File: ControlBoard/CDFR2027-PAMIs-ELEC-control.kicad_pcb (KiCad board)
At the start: 4 copper layers, 96.8 x 76.6 mm, 92 parts, among them J1 Conn_01x04_Pin, Q1 PMOS, U1 USBLC6-2P6

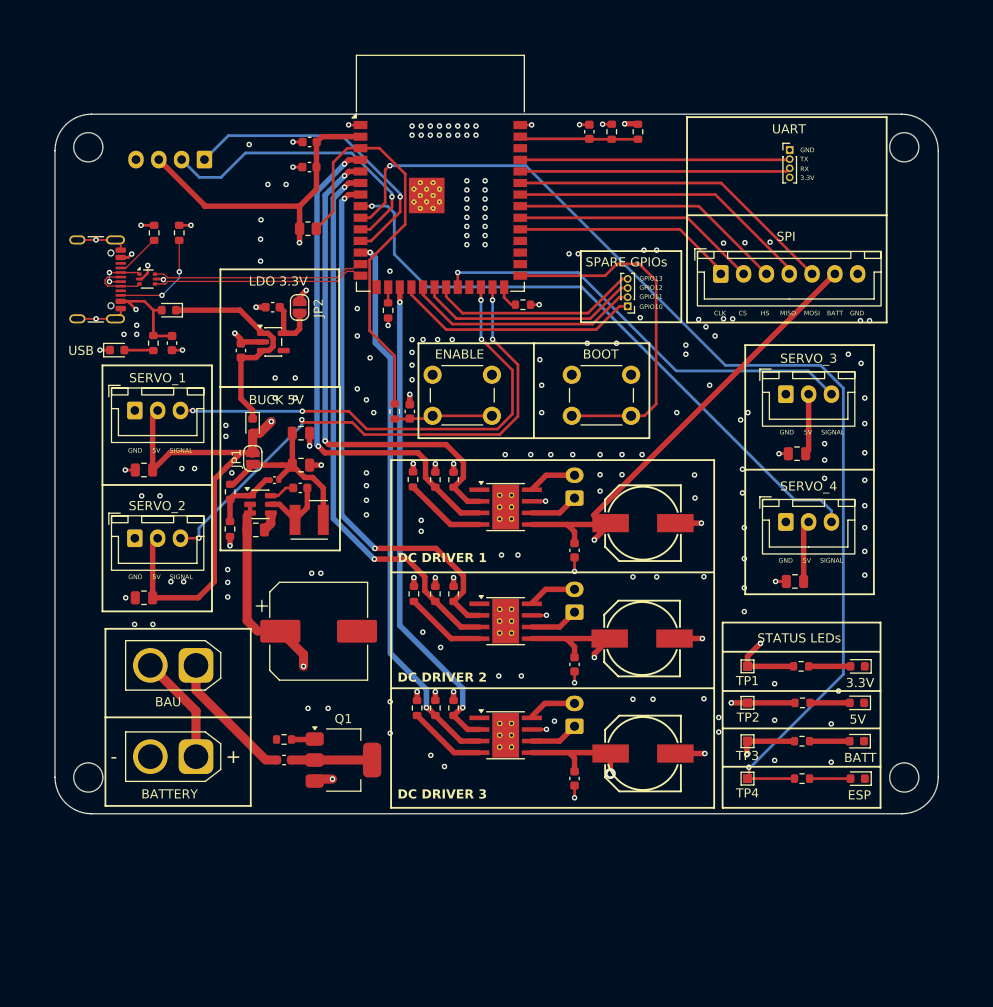
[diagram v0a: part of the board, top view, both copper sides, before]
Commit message: (feat): routing v2
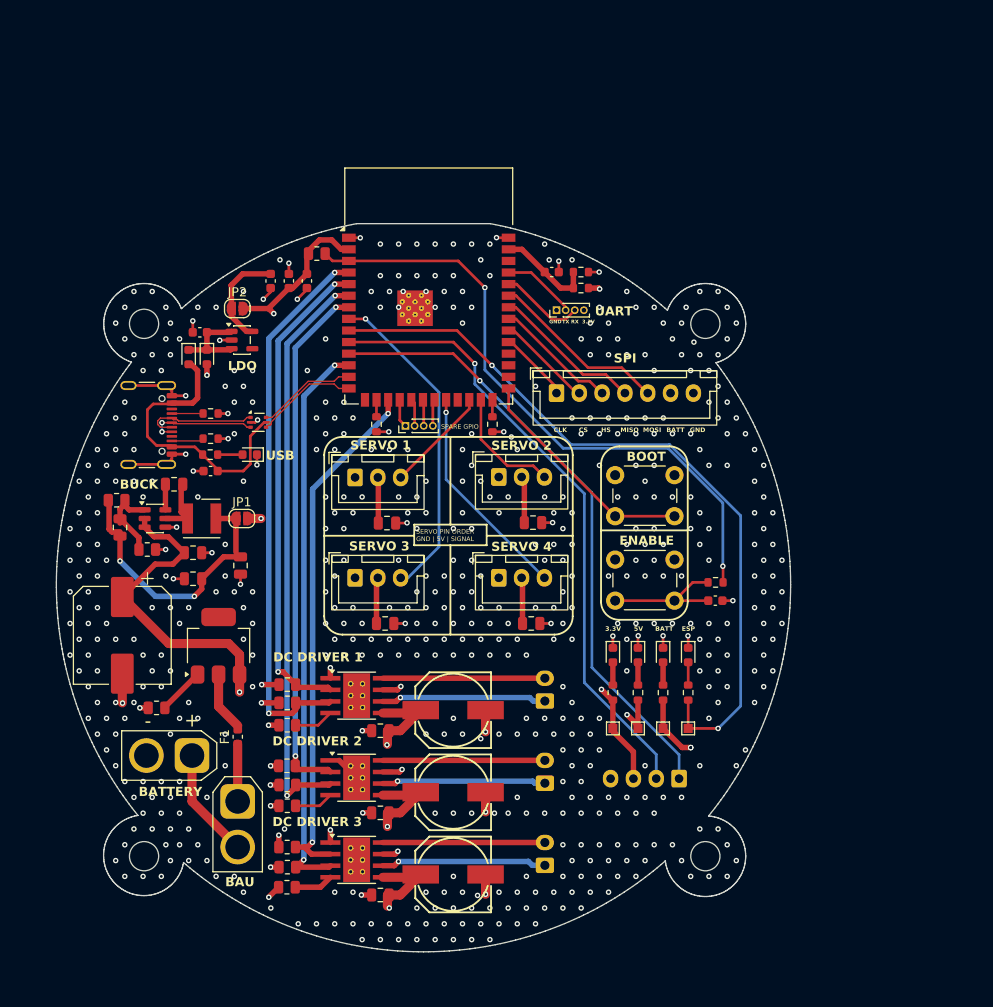
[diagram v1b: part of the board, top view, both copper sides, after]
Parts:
- C13, C15, C17, C7: footprint Capacitor_SMD:C_0603_1608Metric -> Capacitor_SMD:C_0805_2012Metric
- C19: footprint Capacitor_SMD:C_0402_1005Metric -> Capacitor_SMD:C_0805_2012Metric
- R10, R11, R12, R13, R14, R15, R16, R17, R5, R9: footprint Resistor_SMD:R_0603_1608Metric -> Resistor_SMD:R_0805_2012Metric
- R18, R19: footprint PCM_SparkFun-Resistor:R_0603_1608Metric -> Resistor_SMD:R_0805_2012Metric
- moved H4 97.0 mm to (93.6, 85.7)
- moved I2C1 85.5 mm to (152.2, 135.5)
- moved H3 83.9 mm to (155.1, 85.7)
- moved H2 80.7 mm to (155.1, 144.0)
- moved H1 77.9 mm to (93.6, 144.0)
- moved SERVO_4 47.6 mm to (116.8, 113.5)
- moved C23 45.1 mm to (120.0, 118.5), turned to 0 degrees
- moved REF** 43.7 mm to (124.5, 108.6)
- moved C21 43.4 mm to (136.2, 107.5), turned to 0 degrees
- moved SERVO_2 40.4 mm to (132.5, 102.5)
- moved R1 39.8 mm to (156.2, 114.0), turned to 0 degrees
- moved C1 39.4 mm to (156.2, 116.0), turned to 180 degrees
- moved SERVO_3 37.3 mm to (132.5, 113.5)
- moved C22 34.6 mm to (136.1, 118.5), turned to 0 degrees
- moved UART1 31.0 mm to (138.8, 84.2), turned to 90 degrees
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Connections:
- net Net-(U1-I/O1-Pad1) renamed /External IO/D-
- net Net-(U1-I/O2-Pad3) renamed /External IO/D+
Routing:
- net +3.3V: track 179.3 -> 106.9 mm, vias 3 -> 2
- net BATT: track 310.3 -> 245.7 mm
- net +5V: track 176.1 -> 119.9 mm, vias 2 -> 3
- net /Actuators & Utility/SERVO_2: track 60.4 -> 13.0 mm, vias 4 -> 0
- net /Actuators & Utility/SERVO_1: track 53.2 -> 11.6 mm, vias 4 -> 0
- net /Actuators & Utility/STATUS_LED: track 119.6 -> 82.1 mm
- net /External IO/SDA: track 32.7 -> 68.5 mm
- net /External IO/SCL: track 32.8 -> 68.2 mm
- net /Actuators & Utility/SERVO_4: track 69.3 -> 35.7 mm
- net /Actuators & Utility/SERVO_3: track 48.1 -> 24.0 mm
- net /Actuators & Utility/GPIO10: track 27.2 -> 3.11 mm
- net /Actuators & Utility/GPIO11: track 26.3 -> 3.00 mm
- net Net-(ESP32-S3-WROOM1-EN): track 45.9 -> 68.9 mm, vias 0 -> 2
- net /Actuators & Utility/GPIO12: track 24.7 -> 2.89 mm
- net /External IO/TXD0: track 29.6 -> 8.16 mm
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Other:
- board size 96.8 x 76.6 mm -> 80.4 x 79.8 mm
- board text added: "BUCK"
- board text added: "Carte de contrôle V2 PAMIs CDFR 2027"
- board text added: "I2C"
- board text added: "LDO"
- board text added: "SERVO 1"
- board text added: "SERVO 2"
- board text added: "SERVO 3"
- board text added: "SERVO 4"
- board text added: "SERVO PIN ORDER GND | 5V | SIGNAL"
- board text added: "SPARE GPIO"
- board text removed: "BUCK 5V"
- board text removed: "Carte de contrôle V1 PAMIs CDFR 2027"
- board text removed: "GPIO10"
- board text removed: "GPIO11"
- board text removed: "GPIO12"
- board text removed: "GPIO13"
- board text removed: "I2C OTOS"
- board text removed: "LDO 3.3V"
- board text removed: "OUT1"
- board text removed: "OUT2"
- board text removed: "SIGNAL"
- board text removed: "SPARE GPIOs"
- board text removed: "STATUS LEDs"
